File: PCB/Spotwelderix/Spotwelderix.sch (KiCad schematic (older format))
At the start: 63 parts, among them IC1 IXDD604SIA, IC2 IXDD604SIA, J1 OnOffTast, J2 probe+, J3 XT90, J4 probe-, J6 XT90, P1 CONN_01X09, Q1 IRFB7430, Q10 FQP27P06, Q11 DMG3402_SOT23_n_Fet_3A, Q12 DMG3402_SOT23_n_Fet_3A, Q2 IRFB7430, Q3 IRFB7430, Q4 IRFB7430, Q5 IRFB7430, Q6 IRFB7430, Q7 IRFB7430, Q8 IRFB7430, Q9 BC817, U1 DS18B20, U2 AD8209, U3 AD8209

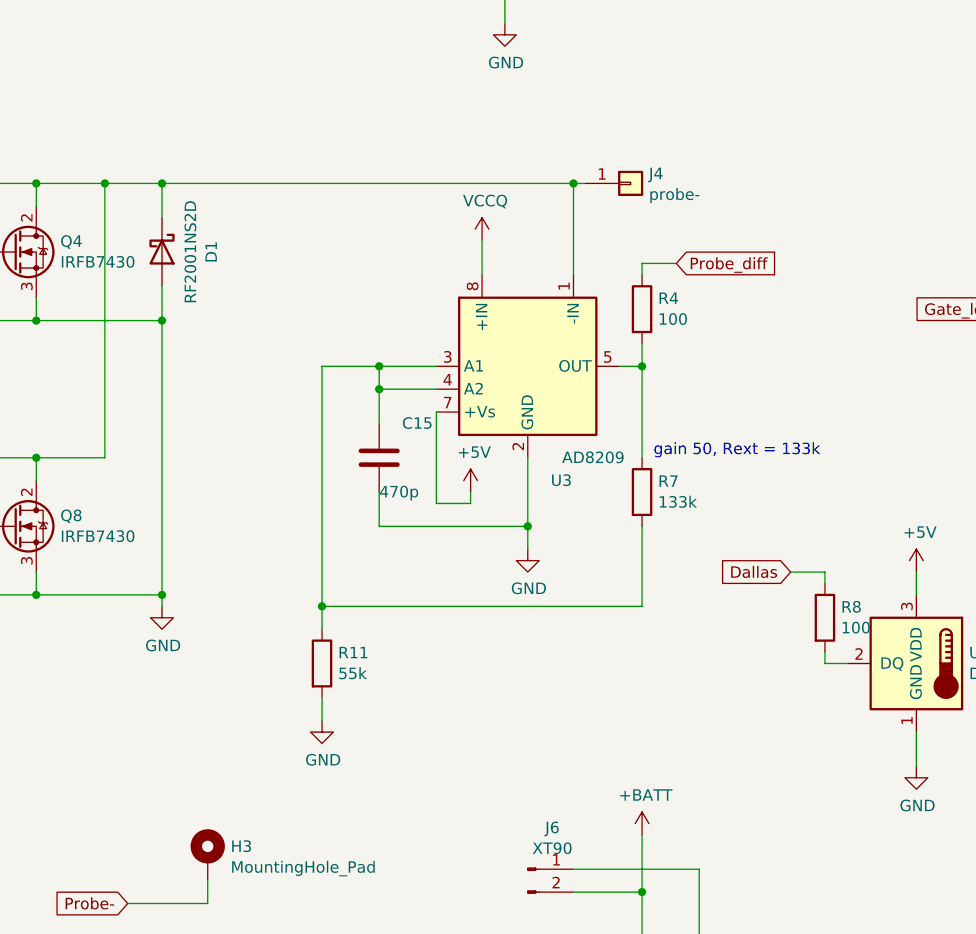
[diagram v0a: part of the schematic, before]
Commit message: auto weld, non functional
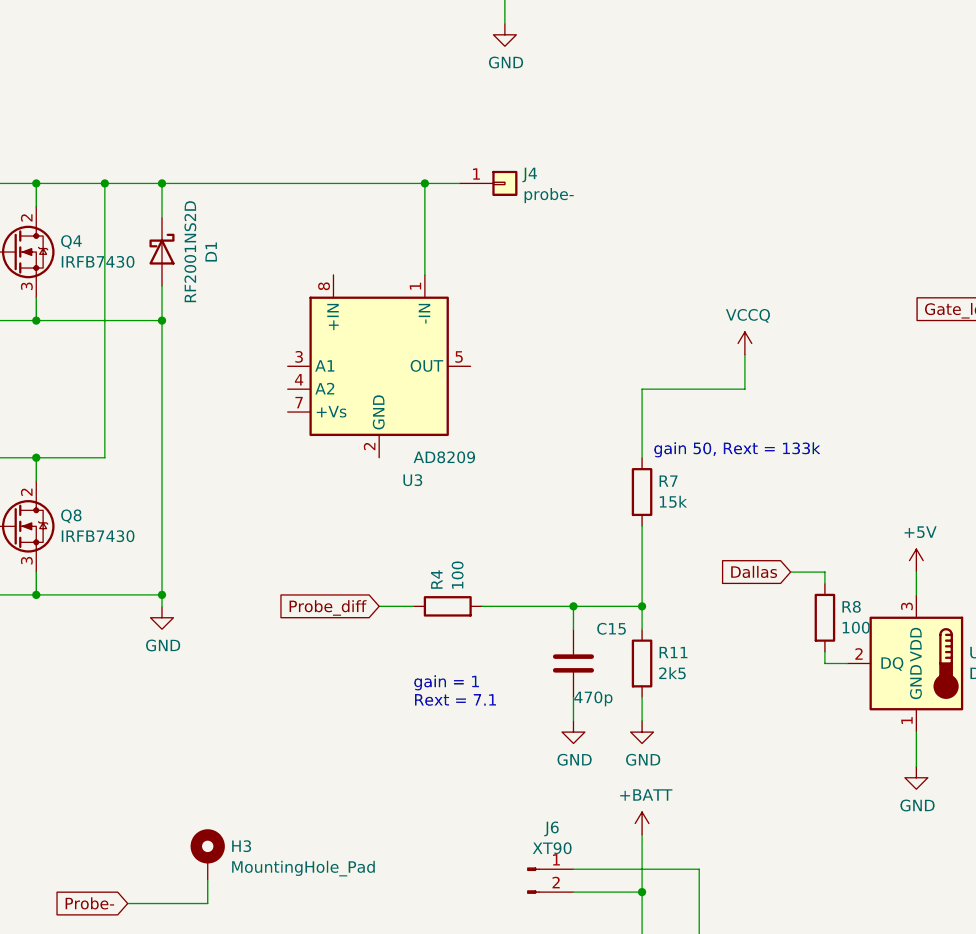
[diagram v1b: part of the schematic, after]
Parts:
- R11: value 55k -> 2k5
- R7: value 133k -> 15k
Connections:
- net +5V: no longer U3.7 (+Vs)
- net GND: no longer U3.2 (GND)
- net VCCQ: now also R7.1; no longer U3.8 (+IN)
- net at C15.1, R11.1, R7.2: now also R4.2; no longer U3.3 (A1), U3.4 (A2)
- now unconnected: U3.5 (OUT)
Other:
- note added: "gain = 1\nRext = 7.1"
- moved on the sheet: C15, J4, R11, R4, U3
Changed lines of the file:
@@
 L Connector_Generic:Conn_01x01 J4
 U 1 1 6027240D
-P 6300 3550
-F 0 "J4" H 6380 3592 50  0000 L CNN
-F 1 "probe-" H 6380 3501 50  0000 L CNN
-F 2 "MountingHole:MountingHole_5.3mm_M5_Pad_Via" H 6300 3550 50  0001 C CNN
-F 3 "~" H 6300 3550 50  0001 C CNN
-	1    6300 3550
+P 5750 3550
+F 0 "J4" H 5830 3592 50  0000 L CNN
+F 1 "probe-" H 5830 3501 50  0000 L CNN
+F 2 "MountingHole:MountingHole_5.3mm_M5_Pad_Via" H 5750 3550 50  0001 C CNN
+F 3 "~" H 5750 3550 50  0001 C CNN
+	1    5750 3550
 	1    0    0    -1
 $EndComp
@@
 	1    0    0    -1
 $EndComp
-Wire Wire Line
-	6100 3550 6050 3550
 Connection ~ 4250 3550
 Wire Wire Line
@@
 L Amplifier_Current:AD8209 U3
 U 1 1 61E0AEFA
-P 5850 4350
-F 0 "U3" H 5950 3850 50  0000 L CNN
-F 1 "AD8209" H 6000 3950 50  0000 L CNN
-F 2 "Package_SO:MSOP-8_3x3mm_P0.65mm" H 5900 4000 50  0001 L CNN
-F 3 "https://www.analog.com/media/en/technical-documentation/data-sheets/AD8209.pdf" H 6500 3650 50  0001 C CNN
-	1    5850 4350
+P 5200 4350
+F 0 "U3" H 5300 3850 50  0000 L CNN
+F 1 "AD8209" H 5350 3950 50  0000 L CNN
+F 2 "Package_SO:MSOP-8_3x3mm_P0.65mm" H 5250 4000 50  0001 L CNN
+F 3 "https://www.analog.com/media/en/technical-documentation/data-sheets/AD8209.pdf" H 5850 3650 50  0001 C CNN
+	1    5200 4350
 	1    0    0    -1
 $EndComp
@@
 L power:VCCQ #PWR0114
 U 1 1 61E1E268
-P 5650 3800
-F 0 "#PWR0114" H 5650 3650 50  0001 C CNN
-F 1 "VCCQ" H 5665 3973 50  0000 C CNN
-F 2 "" H 5650 3800 50  0001 C CNN
-F 3 "" H 5650 3800 50  0001 C CNN
-	1    5650 3800
-	1    0    0    -1
-$EndComp
-Wire Wire Line
-	5650 3950 5650 3800
-Wire Wire Line
-	6050 3950 6050 3550
+P 6800 4300
+F 0 "#PWR0114" H 6800 4150 50  0001 C CNN
+F 1 "VCCQ" H 6815 4473 50  0000 C CNN
+F 2 "" H 6800 4300 50  0001 C CNN
+F 3 "" H 6800 4300 50  0001 C CNN
+	1    6800 4300
+	1    0    0    -1
+$EndComp
+Wire Wire Line
+	6800 4450 6800 4300
 $Comp
 L power:GND #PWR0118
@@
 Wire Wire Line
 	7000 1050 8900 1050
-Text GLabel 6500 3900 2    50   Input ~ 0
+Text GLabel 5200 5400 0    50   Input ~ 0
 Probe_diff
 Text GLabel 2100 6900 0    50   Input ~ 0
@@
 L Arduino_Spot_Welderparts:R R4
 U 1 1 6202236D
-P 6350 4100
-F 0 "R4" H 6420 4146 50  0000 L CNN
-F 1 "100" H 6420 4055 50  0000 L CNN
-F 2 "Resistor_SMD:R_0805_2012Metric" H 6420 4009 50  0001 L CNN
-F 3 "" H 6350 4100 50  0000 C CNN
-	1    6350 4100
-	1    0    0    -1
-$EndComp
-Wire Wire Line
-	6250 4350 6350 4350
-Wire Wire Line
-	6350 4350 6350 4250
-Wire Wire Line
-	6350 3950 6350 3900
-Wire Wire Line
-	6350 3900 6500 3900
+P 5500 5400
+F 0 "R4" H 5570 5446 50  0000 L CNN
+F 1 "100" H 5570 5355 50  0000 L CNN
+F 2 "Resistor_SMD:R_0805_2012Metric" H 5570 5309 50  0001 L CNN
+F 3 "" H 5500 5400 50  0000 C CNN
+	1    5500 5400
+	0    -1   -1   0
+$EndComp
+Wire Wire Line
+	5350 5400 5200 5400
 $Comp
 L power:GND #PWR0123
 U 1 1 62054793
-P 5850 5150
-F 0 "#PWR0123" H 5850 4900 50  0001 C CNN
-F 1 "GND" H 5855 4977 50  0000 C CNN
-F 2 "" H 5850 5150 50  0001 C CNN
-F 3 "" H 5850 5150 50  0001 C CNN
-	1    5850 5150
-	1    0    0    -1
-$EndComp
-Wire Wire Line
-	5850 5150 5850 5050
-Wire Wire Line
-	5200 5050 5850 5050
-Connection ~ 5850 5050
-Wire Wire Line
-	5850 5050 5850 4750
-Connection ~ 6050 3550
-Wire Wire Line
-	4250 3550 6050 3550
+P 6050 5900
+F 0 "#PWR0123" H 6050 5650 50  0001 C CNN
+F 1 "GND" H 6055 5727 50  0000 C CNN
+F 2 "" H 6050 5900 50  0001 C CNN
+F 3 "" H 6050 5900 50  0001 C CNN
+	1    6050 5900
+	1    0    0    -1
+$EndComp
 $Comp
 L Device:C C15
 U 1 1 62088B6C
-P 5200 4750
-F 0 "C15" H 5300 4900 50  0000 L CNN
-F 1 "470p" H 5200 4600 50  0000 L CNN
-F 2 "Capacitor_SMD:C_0805_2012Metric_Pad1.18x1.45mm_HandSolder" H 5238 4600 50  0001 C CNN
-F 3 "https://www.mouser.de/ProductDetail/Samsung-Electro-Mechanics/CL31A106KBHNNNE/?qs=sGAEpiMZZMuMW9TJLBQkXpvci%252BYHLlg21rnqFxf28Ww%3D" H 5200 4750 50  0001 C CNN
-	1    5200 4750
-	1    0    0    -1
-$EndComp
-Wire Wire Line
-	5450 4450 5200 4450
-Wire Wire Line
-	5200 4450 5200 4350
-Wire Wire Line
-	5200 4350 5450 4350
-Wire Wire Line
-	5200 4450 5200 4600
-Connection ~ 5200 4450
-Wire Wire Line
-	5200 4900 5200 5050
-$Comp
-L power:+5V #PWR0124
-U 1 1 6209AE8B
-P 5600 4900
-F 0 "#PWR0124" H 5600 4750 50  0001 C CNN
-F 1 "+5V" H 5615 5073 50  0000 C CNN
-F 2 "" H 5600 4900 50  0001 C CNN
-F 3 "" H 5600 4900 50  0001 C CNN
-	1    5600 4900
-	1    0    0    -1
-$EndComp
-Wire Wire Line
-	5450 4950 5600 4950
-Wire Wire Line
-	5600 4950 5600 4900
-Wire Wire Line
-	5450 4550 5450 4950
+P 6050 5650
+F 0 "C15" H 6150 5800 50  0000 L CNN
+F 1 "470p" H 6050 5500 50  0000 L CNN
+F 2 "Capacitor_SMD:C_0805_2012Metric_Pad1.18x1.45mm_HandSolder" H 6088 5500 50  0001 C CNN
+F 3 "https://www.mouser.de/ProductDetail/Samsung-Electro-Mechanics/CL31A106KBHNNNE/?qs=sGAEpiMZZMuMW9TJLBQkXpvci%252BYHLlg21rnqFxf28Ww%3D" H 6050 5650 50  0001 C CNN
+	1    6050 5650
+	1    0    0    -1
+$EndComp
 Text Notes 6400 4750 0    50   ~ 0
 gain 50, Rext = 133k\n
@@
 P 6350 4900
 F 0 "R7" H 6420 4946 50  0000 L CNN
-F 1 "133k" H 6420 4855 50  0000 L CNN
+F 1 "15k" H 6420 4855 50  0000 L CNN
 F 2 "Resistor_SMD:R_0805_2012Metric" H 6420 4809 50  0001 L CNN
 F 3 "" H 6350 4900 50  0000 C CNN
@@
 	6350 5050 6350 5400
 Wire Wire Line
-	6350 5400 4950 5400
-Wire Wire Line
-	4950 5400 4950 4350
-Wire Wire Line
-	4950 4350 5200 4350
-Connection ~ 5200 4350
-Wire Wire Line
-	6350 4750 6350 4350
-Connection ~ 6350 4350
+	6350 5400 6050 5400
+Wire Wire Line
+	6350 4750 6350 4450
 $Comp
 L my_parts:DMG3402_SOT23_n_Fet_3A Q12
@@
 L Arduino_Spot_Welderparts:R R11
 U 1 1 619FF475
-P 4950 5650
-F 0 "R11" H 5020 5696 50  0000 L CNN
-F 1 "55k" H 5020 5605 50  0000 L CNN
-F 2 "Resistor_SMD:R_0805_2012Metric" H 5020 5559 50  0001 L CNN
-F 3 "" H 4950 5650 50  0000 C CNN
-	1    4950 5650
+P 6350 5650
+F 0 "R11" H 6420 5696 50  0000 L CNN
+F 1 "2k5" H 6420 5605 50  0000 L CNN
+F 2 "Resistor_SMD:R_0805_2012Metric" H 6420 5559 50  0001 L CNN
+F 3 "" H 6350 5650 50  0000 C CNN
+	1    6350 5650
 	1    0    0    -1
 $EndComp
@@
 L power:GND #PWR08
 U 1 1 61A13350
-P 4950 5900
-F 0 "#PWR08" H 4950 5650 50  0001 C CNN
-F 1 "GND" H 4955 5727 50  0000 C CNN
-F 2 "" H 4950 5900 50  0001 C CNN
-F 3 "" H 4950 5900 50  0001 C CNN
-	1    4950 5900
-	1    0    0    -1
-$EndComp
-Wire Wire Line
-	4950 5500 4950 5400
-Connection ~ 4950 5400
-Wire Wire Line
-	4950 5900 4950 5800
+P 6350 5900
+F 0 "#PWR08" H 6350 5650 50  0001 C CNN
+F 1 "GND" H 6355 5727 50  0000 C CNN
+F 2 "" H 6350 5900 50  0001 C CNN
+F 3 "" H 6350 5900 50  0001 C CNN
+	1    6350 5900
+	1    0    0    -1
+$EndComp
+Wire Wire Line
+	6350 5500 6350 5400
+Wire Wire Line
+	6350 5900 6350 5800
+Text Notes 5350 5850 0    50   ~ 0
+gain = 1\nRext = 7.1
+Wire Wire Line
+	6050 5900 6050 5800
+Wire Wire Line
+	6050 5500 6050 5400
+Wire Wire Line
+	6800 4450 6350 4450
+Wire Wire Line
+	5400 3950 5400 3550
+Wire Wire Line
+	4250 3550 5400 3550
+Wire Wire Line
+	5550 3550 5400 3550
+Connection ~ 5400 3550
+Connection ~ 6350 5400
+Wire Wire Line
+	5650 5400 6050 5400
+Connection ~ 6050 5400
 $EndSCHEMATC
